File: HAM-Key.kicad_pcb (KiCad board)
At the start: 2 copper layers, 60.2 x 57.7 mm, 29 parts, among them J2 Conn_01x04, Q1 DTC143Z, SW1 SW_Push, SW2 SW_SPDT, SW3 SW_SPDT, SW4 SW_SPDT

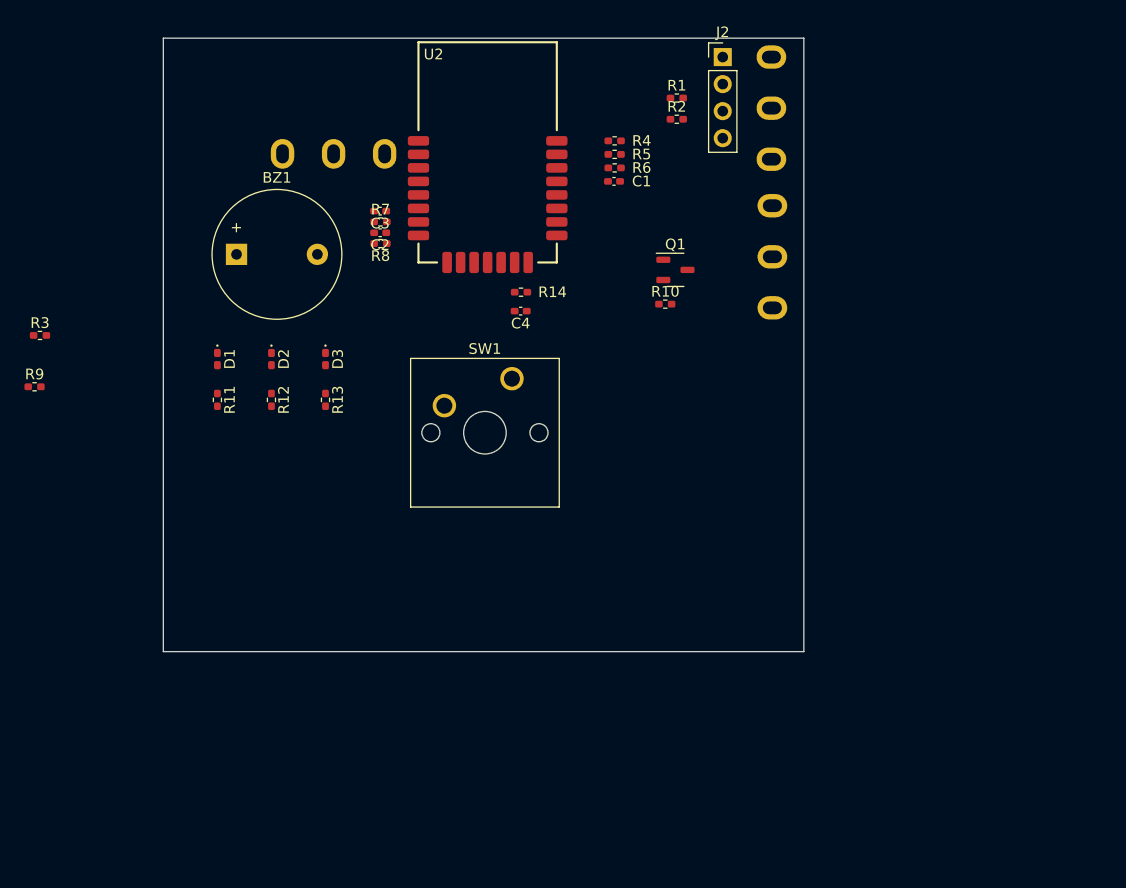
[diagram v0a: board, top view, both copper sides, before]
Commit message: update
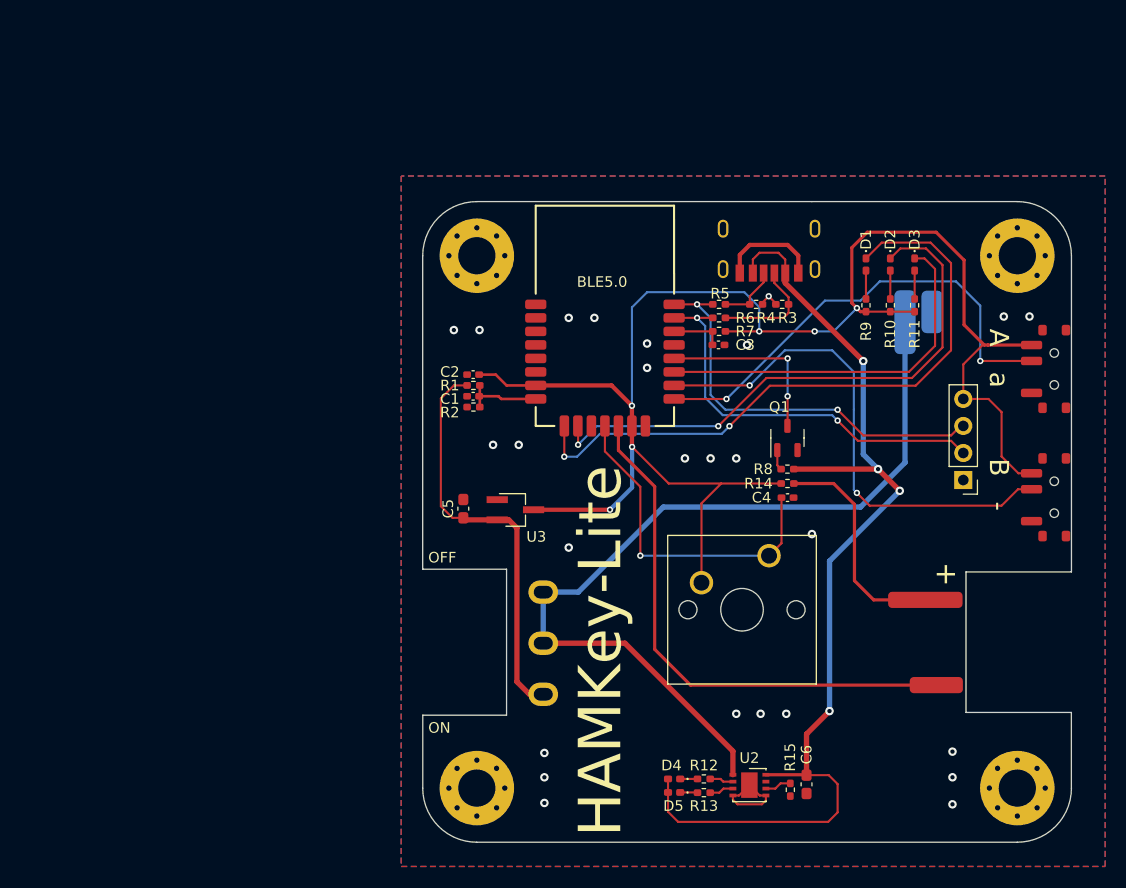
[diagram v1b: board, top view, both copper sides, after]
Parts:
- removed the R9 at (80.1, 87.6)
- added BATT1: Battery_Cell, nigh_Library:BATT2030, B.Cu at (128.4, 78.5)
- added C5: 1uF, Capacitor_SMD:C_0603_1608Metric_Pad1.08x0.95mm_HandSolder, F.Cu at (120.4, 99.1)
- added C6: 1uF, Capacitor_SMD:C_0603_1608Metric_Pad1.08x0.95mm_HandSolder, F.Cu at (152.7, 125.0)
- added D4: BLUE, LED_SMD:LED_0402_1005Metric_Pad0.77x0.64mm_HandSolder, F.Cu at (140.2, 124.5)
- added D5: RED, LED_SMD:LED_0402_1005Metric_Pad0.77x0.64mm_HandSolder, F.Cu at (140.2, 125.8)
- added H1: M3.5, MountingHole:MountingHole_3.5mm_Pad_Via, F.Cu at (121.7, 75.3)
- added H2: M3.5, MountingHole:MountingHole_3.5mm_Pad_Via, F.Cu at (172.5, 75.3)
- added H3: M3.5, MountingHole:MountingHole_3.5mm_Pad_Via, F.Cu at (121.7, 125.3)
- added H4: M3.5, MountingHole:MountingHole_3.5mm_Pad_Via, F.Cu at (172.5, 125.3)
- added R12: 1k, Resistor_SMD:R_0402_1005Metric_Pad0.72x0.64mm_HandSolder, F.Cu at (143.0, 124.5)
- added R13: 1k, Resistor_SMD:R_0402_1005Metric_Pad0.72x0.64mm_HandSolder, F.Cu at (143.0, 125.8)
- added U2: ~, Package_DFN_QFN:DFN-8-1EP_3x3mm_P0.65mm_EP1.55x2.4mm, F.Cu at (147.3, 125.1)
- added U3: ~, Package_TO_SOT_SMD:TSOT-23_HandSoldering, F.Cu at (125.3, 99.2)
- added USB1: USB_C_Receptacle_PowerOnly_6P, nigh_Library:Type-C-3.2H, F.Cu at (149.1, 77.7)
- BZ1: footprint Buzzer_Beeper:Buzzer_12x9.5RM7.6 -> nigh_Library:buzzer_SMD
- D1: value LED -> RED
- D2: value LED -> BLUE
- D3: value LED -> WHITE
- R14: value 330R -> 0R
- R15: renamed from R3; value X -> 10k
- SW3: renamed from SW2; footprint nigh_Library:SS12D06G5 -> nigh_Library:MSK12
- SW4: renamed from SW3; footprint nigh_Library:SS12D06G5 -> nigh_Library:MSK12
- moved R15 82.4 mm to (151.1, 125.5), turned to -90 degrees
- moved BZ1 75.6 mm to (167.4, 107.7), turned to -90 degrees
- moved D1 61.6 mm to (158.2, 76.1)
- moved R9 61.6 mm to (158.2, 80.0)
- moved D2 58.8 mm to (160.5, 76.1)
- moved R10 58.8 mm to (160.5, 80.0)
- moved R11 56.1 mm to (162.8, 80.0)
- moved D3 56.1 mm to (162.8, 76.1)
- moved SW2 50.0 mm to (127.9, 111.7), turned to 90 degrees
- moved J2 45.7 mm to (167.4, 96.4), turned to 180 degrees
- moved SW4 36.2 mm to (175.9, 86.0)
- moved SW3 34.8 mm to (175.9, 98.0)
- moved R14 30.8 mm to (150.9, 96.7)
- moved C4 30.6 mm to (150.9, 98.0)
- moved SW1 29.3 mm to (149.1, 103.5)
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- renumbered C2 to C1, C3 to C2, C1 to C3, R7 to R1, R12 to R10, R13 to R11, R8 to R2, R1 to R3, R2 to R4, R4 to R5, R5 to R6, R6 to R7, R10 to R8, R11 to R9, SW4 to SW2, U2 to U1
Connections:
- R5 pad 2: /CC1 -> /CC2
- R6 pad 2: /CC2 -> /CC1
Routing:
- net +3.3V: track 0.00 -> 151.8 mm, vias 0 -> 6
- net +5V: track 0.00 -> 99.7 mm, vias 0 -> 4
- net Net-(BATT1-+): track 0.00 -> 81.3 mm
- net /LED_RED: track 0.00 -> 61.0 mm, vias 0 -> 2
- net /LED_BLUE: track 0.00 -> 53.5 mm, vias 0 -> 2
- net /BUZZER: track 0.00 -> 50.3 mm
- net /SW1: track 0.00 -> 48.1 mm, vias 0 -> 2
- net /SW2: track 0.00 -> 44.3 mm, vias 0 -> 2
- net /BAT+: track 0.00 -> 38.5 mm
- net /SWDIO: track 0.00 -> 38.4 mm, vias 0 -> 2
- net /SWDCLK: track 0.00 -> 37.9 mm, vias 0 -> 2
- net /LED_WHITE: track 0.00 -> 35.1 mm
- net /BTN: track 0.00 -> 31.6 mm, vias 0 -> 1
- net Net-(BZ1--): track 0.00 -> 21.1 mm
- net GND: track 0.00 -> 19.9 mm, vias 0 -> 26
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- added copper zone on B.Cu, net GND
- added copper zone on F.Cu, net GND
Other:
- board size 60.2 x 57.7 mm -> 61 x 60.2 mm
- board text added: "A a"
- board text added: "B -"
- board text added: "BLE5.0"
- board text added: "Battery: 3.7V 300mAh Input: 5.0V 200mA"
- board text added: "HAMKey-Lite"
- board text added: "HelloWorks@GitHub"
- board text added: "OFF"
- board text added: "ON"
- board text added: "https://github.com/Nigh/HAM-Key"
